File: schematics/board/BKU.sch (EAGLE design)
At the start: 48 parts

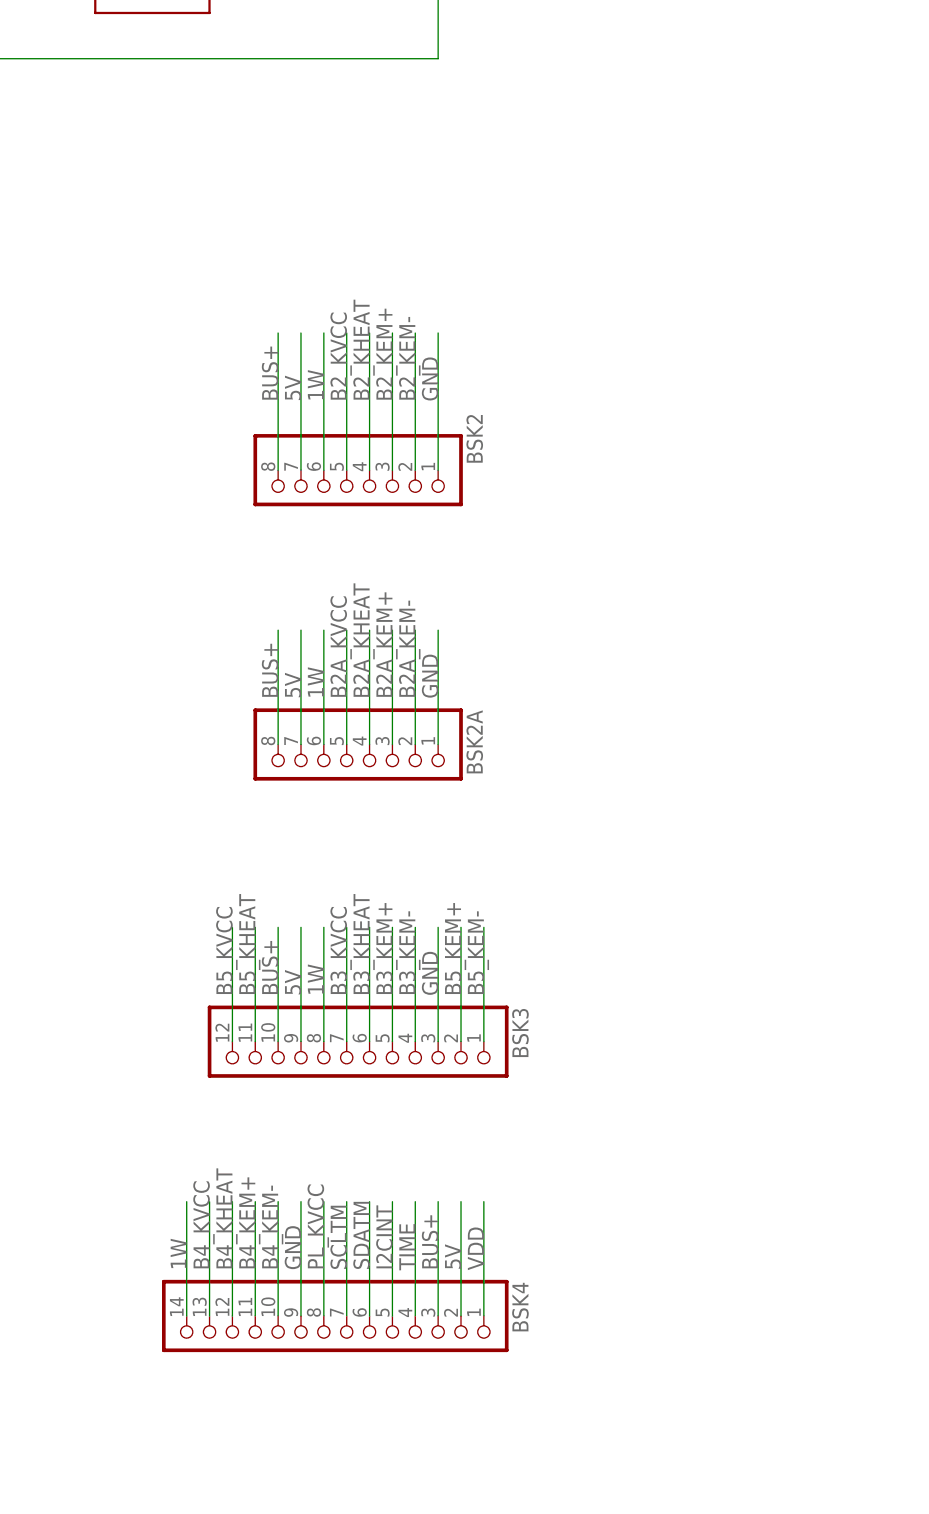
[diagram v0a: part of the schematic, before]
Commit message: Сделаны платы CROSSnew, SPIDERnew, BSK2
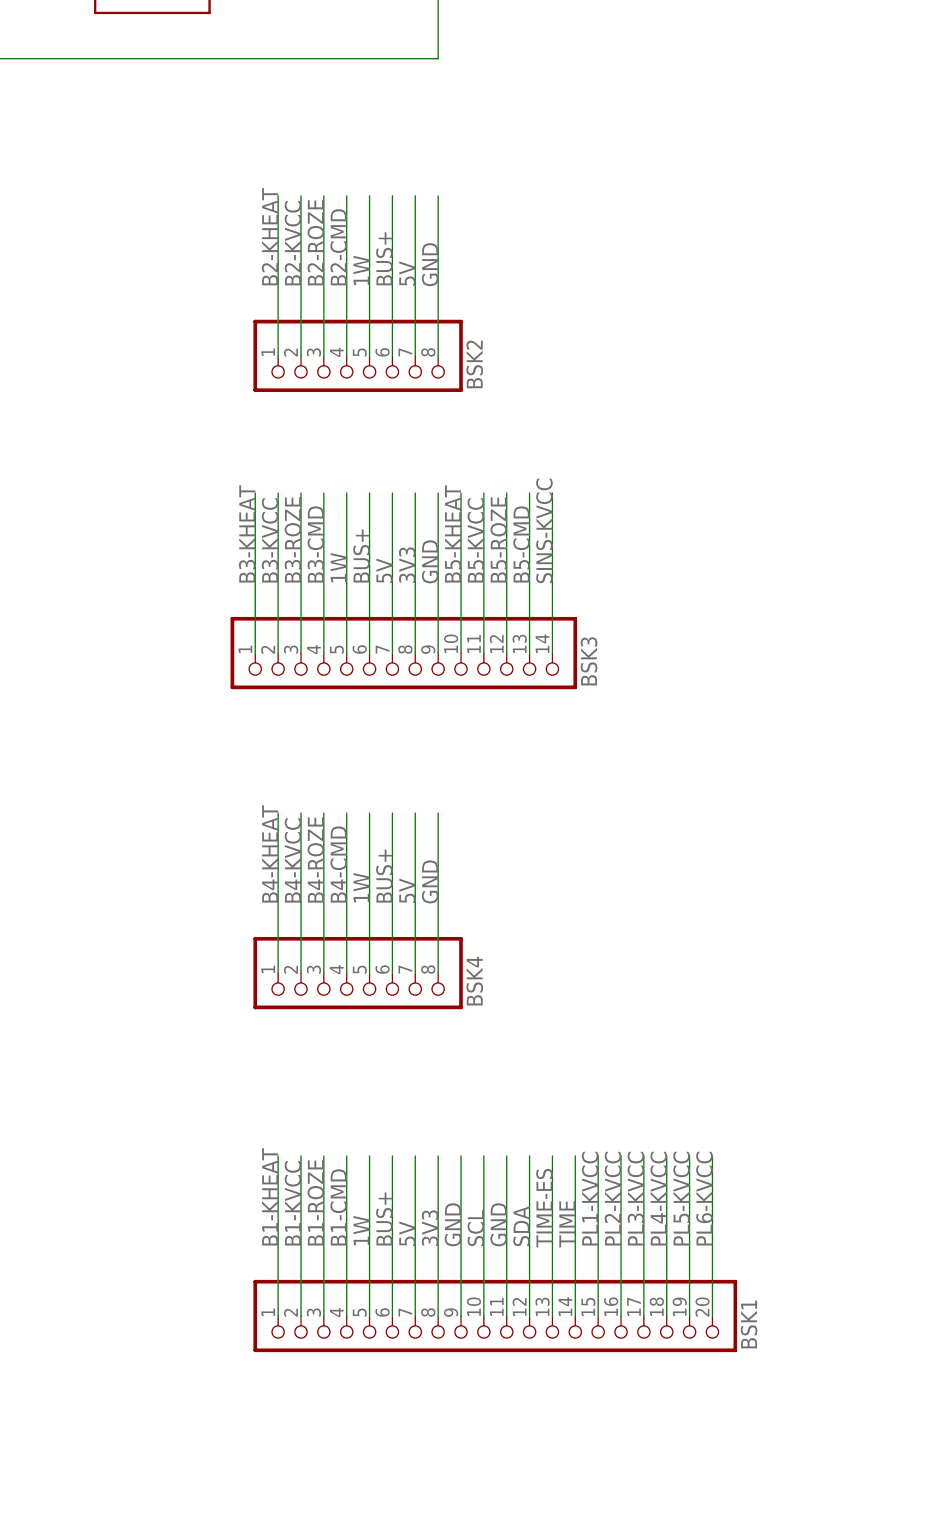
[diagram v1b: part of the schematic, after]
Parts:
- removed BSK2A: (no value), pinheadCS:PINHD-1X8
- added BSK1: (no value), pinheadCS:PINHD-1X20
- BSK3: device pinheadCS:PINHD-1X12 -> pinheadCS:PINHD-1X14
- BSK4: device pinheadCS:PINHD-1X14 -> pinheadCS:PINHD-1X8
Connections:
- new net 3V3: BSK1.8, BSK3.8
- new net B1-CMD: BSK1.4
- new net B1-KHEAT: BSK1.1
- new net B1-KVCC: BSK1.2
- new net B1-ROZE: BSK1.3
- new net B2-CMD: BSK2.4
- new net B2-KHEAT: BSK2.1
- new net B2-KVCC: BSK2.2
- new net B2-ROZE: BSK2.3
- new net B3-CMD: BSK3.4
- new net B3-KHEAT: BSK3.1
- new net B3-KVCC: BSK3.2
- new net B3-ROZE: BSK3.3
- new net B4-CMD: BSK4.4
- new net B4-KHEAT: BSK4.1
- new net B4-KVCC: BSK4.2
- new net B4-ROZE: BSK4.3
- new net B5-CMD: BSK3.13
- new net B5-KHEAT: BSK3.10
- new net B5-KVCC: BSK3.11
- new net B5-ROZE: BSK3.12
- new net PL1-KVCC: BSK1.15
- new net PL2-KVCC: BSK1.16
- new net PL3-KVCC: BSK1.17
- new net PL4-KVCC: BSK1.18
- new net PL5-KVCC: BSK1.19
- new net PL6-KVCC: BSK1.20
- new net SCL: BSK1.10
- new net SDA: BSK1.12
- new net SINS-KVCC: BSK3.14
- net 1W: now also BSK1.5, BSK2.5, BSK3.5, BSK4.5; no longer BSK2.6, BSK2A.6, BSK3.8, BSK4.14
- net 5V: now also BSK1.7, BSK3.7, BSK4.7; no longer BSK2A.7, BSK3.9, BSK4.2
- net B2A_KEM+: no longer BSK2A.3
- net B2A_KEM-: no longer BSK2A.2
- net B2A_KHEAT: no longer BSK2A.4
- net B2A_KVCC: no longer BSK2A.5
- net B2_KEM+: no longer BSK2.3
- net B2_KEM-: no longer BSK2.2
- net B2_KHEAT: no longer BSK2.4
- net B2_KVCC: no longer BSK2.5
- net B3_KEM+: no longer BSK3.5
- net B3_KEM-: no longer BSK3.4
- net B3_KHEAT: no longer BSK3.6
- net B3_KVCC: no longer BSK3.7
- net B4_KEM+: no longer BSK4.11
- net B4_KEM-: no longer BSK4.10
- net B4_KHEAT: no longer BSK4.12
- net B4_KVCC: no longer BSK4.13
- net B5_KEM+: no longer BSK3.2
- net B5_KEM-: no longer BSK3.1
- net B5_KHEAT: no longer BSK3.11
- net B5_KVCC: no longer BSK3.12
- net BUS+: now also BSK1.6, BSK2.6, BSK3.6, BSK4.6; no longer BSK2.8, BSK2A.8, BSK3.10, BSK4.3
- net GND: now also BSK1.11, BSK1.9, BSK2.8, BSK3.9, BSK4.8; no longer BSK2.1, BSK2A.1, BSK3.3, BSK4.9
- net I2CINT: no longer BSK4.5
- net PL_KVCC: no longer BSK4.8
- net SCLTM: no longer BSK4.7
- net SDATM: no longer BSK4.6
- net TIME: now also BSK1.14; no longer BSK4.4
- net TIME-ES: now also BSK1.13
- net VDD: no longer BSK4.1
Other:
- moved on the sheet: BSK2
